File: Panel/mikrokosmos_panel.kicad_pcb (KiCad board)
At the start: 2 copper layers, 200 x 25 mm, 10 parts

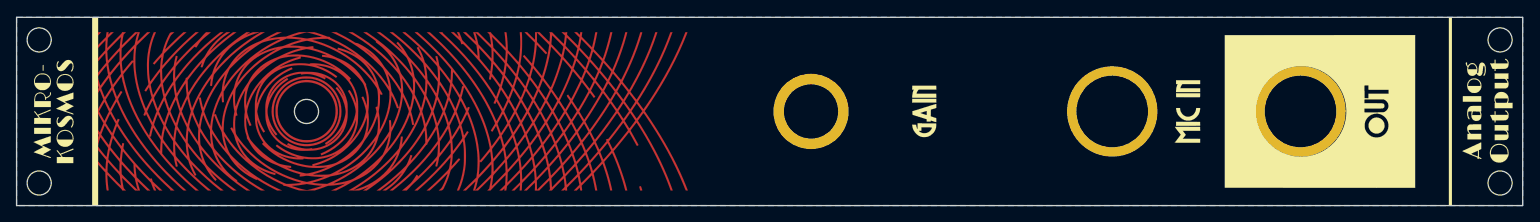
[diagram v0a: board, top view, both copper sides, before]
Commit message: Front Cu fill
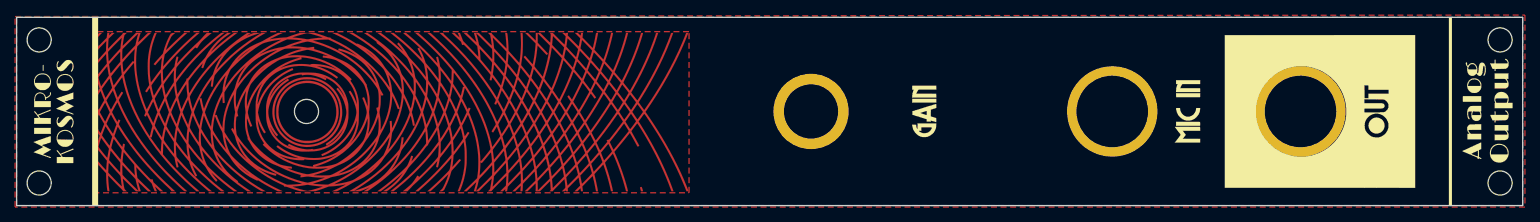
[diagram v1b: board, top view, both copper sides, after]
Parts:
- moved G*** 0.14 mm to (90.6, 92.6)
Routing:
- added copper zone on F.Cu, net GND
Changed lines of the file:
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@@
     (37 F.SilkS user)
     (38 B.Mask user)
-    (39 F.Mask user)
+    (39 F.Mask user hide)
     (40 Dwgs.User user)
     (41 Cmts.User user)
@@
   )
   (module Panel:artc (layer F.Cu)
-    (at 90.5 92.5 90)
+    (at 90.6 92.6 90)
     (fp_text reference G*** (at 0 0 90) (layer F.Cu) hide
       (effects (font (size 1.524 1.524) (thickness 0.3)))
@@
       )
     )
+  )
+  (zone (net 1) (net_name GND) (layer F.Cu) (hatch edge 0.508)
+    (connect_pads (clearance 0.508))
+    (min_thickness 0.254)
+    (fill yes (arc_segments 32) (thermal_gap 0.508) (thermal_bridge_width 0.508))
+    (polygon
+      (pts
+        (xy 250.3 105.2) (xy 49.8 105.2) (xy 49.8 79.9) (xy 250.3 79.7)
+      )
+    )
+    (polygon
+      (pts
+        (xy 60.2 103.3) (xy 139.3 103.3) (xy 139.3 81.9) (xy 60.2 81.9)
+      )
+    )
